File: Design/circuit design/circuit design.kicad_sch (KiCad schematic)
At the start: 22 parts, among them P1 USB_C_Plug_USB2.0, U1 STM32H743VITx, U2 NEO-7M-0, U3 ESP-01, U4 TP4056-42-ESOP8, U5 MP1584EN, U6 MP1584EN

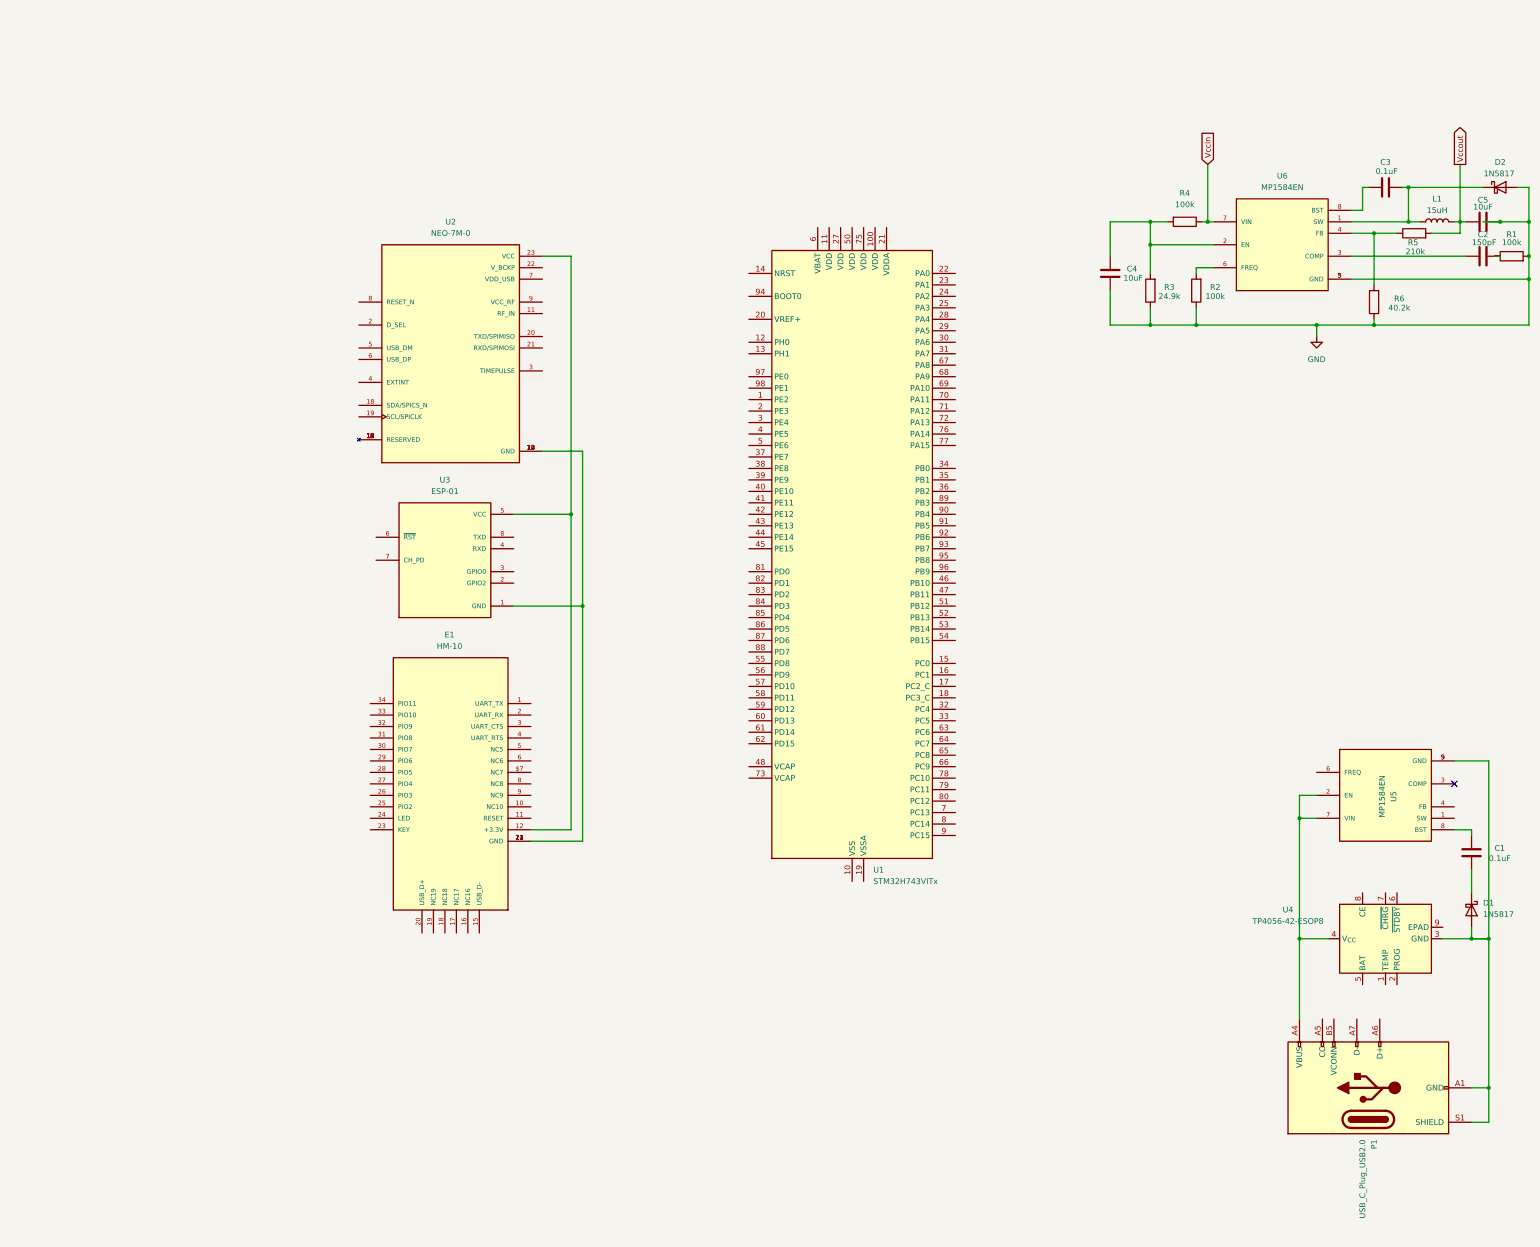
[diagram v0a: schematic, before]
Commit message: [2025-11-20 15:18:30 From Windows 11 Home]: Update
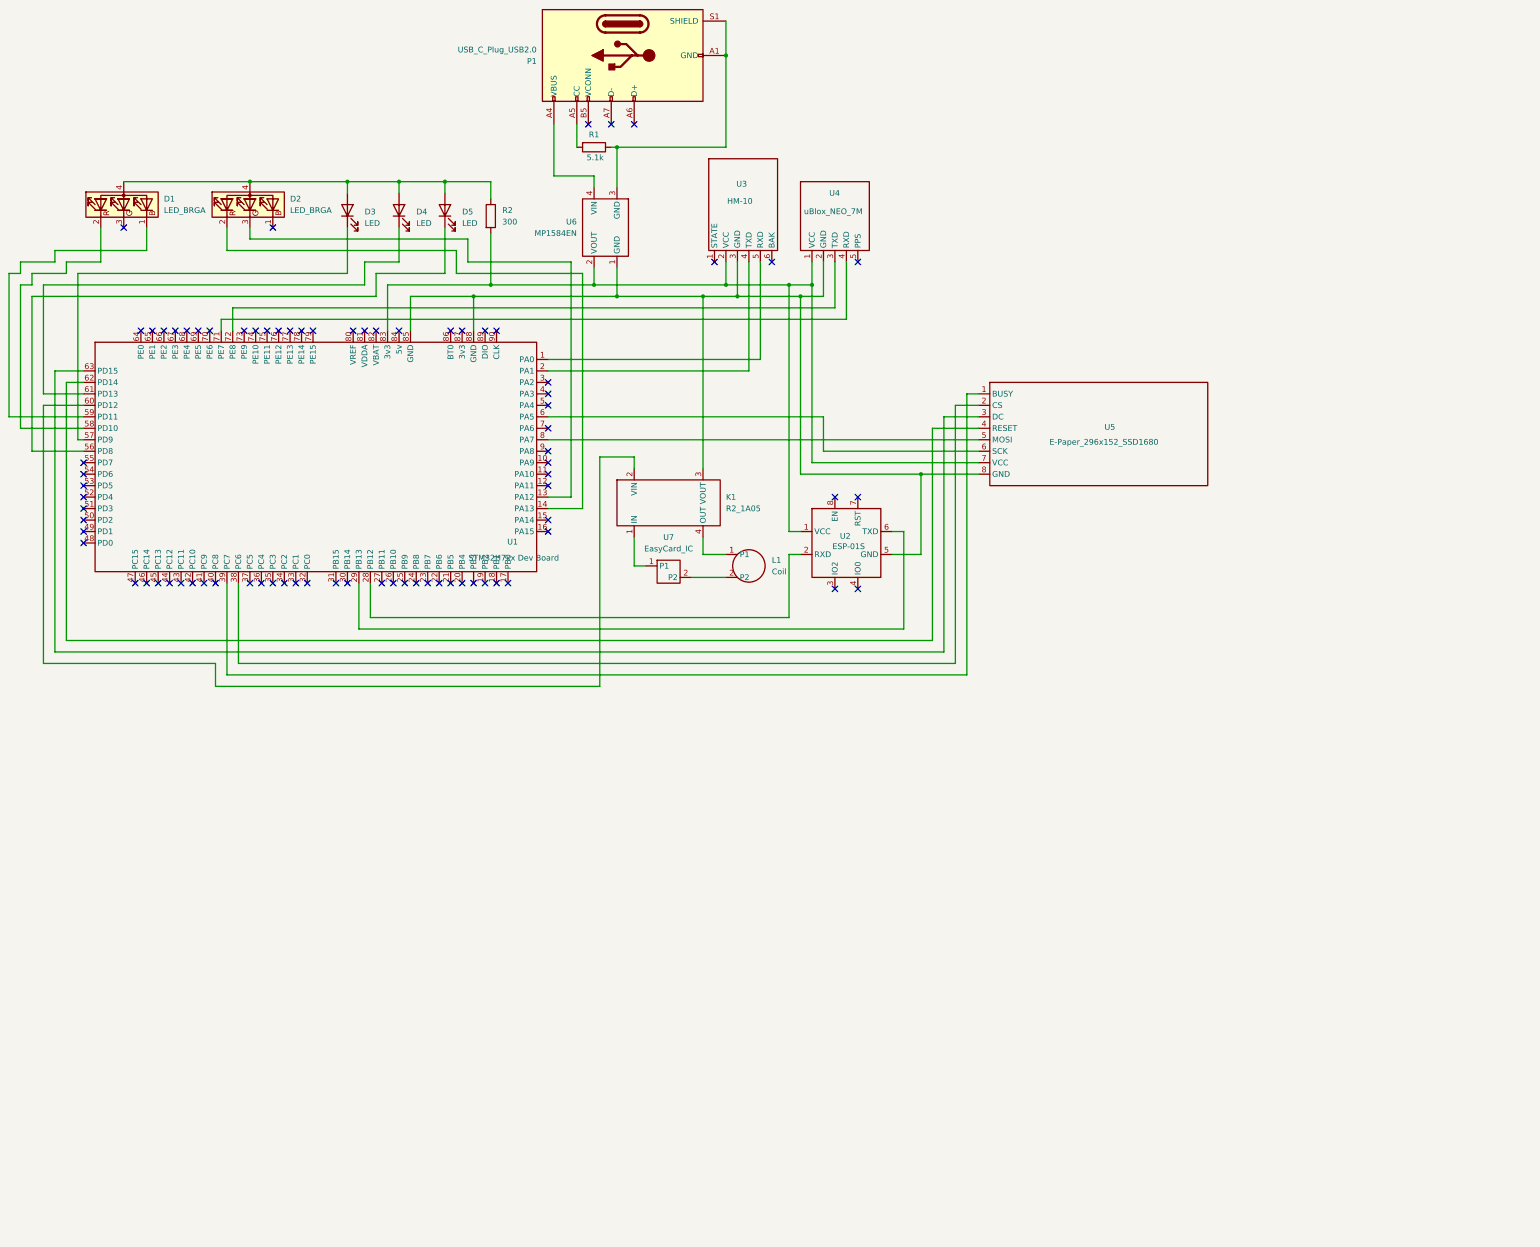
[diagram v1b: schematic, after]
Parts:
- removed C1, C3: 0.1uF, symbol Device:C
- removed C2: 150pF, symbol Device:C
- removed C4, C5: 10uF, symbol Device:C
- removed D1, D2: 1N5817, Diode_THT:D_DO-41_SOD81_P10.16mm_Horizontal, symbol Diode:1N5817
- removed E1: HM-10, HM-10:26.9X13X2.2_BOARD, symbol HM-10:HM-10
- removed L1: 15uH, symbol Device:L
- removed R3: 24.9k, symbol Device:R
- removed R4: 100k, symbol Device:R
- removed R5: 210k, symbol Device:R
- removed R6: 40.2k, symbol Device:R
- removed U1: STM32H743VITx, Package_QFP:LQFP-100_14x14mm_P0.5mm, symbol MCU_ST_STM32H7:STM32H743VITx
- removed U2: NEO-7M-0, NEO-7M-0:XCVR_NEO-7M-0, symbol NEO-7M-0:NEO-7M-0
- removed U3: ESP-01, ESP-01:MODULE_ESP-01, symbol ESP-01:ESP-01
- removed U4: TP4056-42-ESOP8, Package_SO:SOIC-8-1EP_3.9x4.9mm_P1.27mm_EP2.41x3.3mm_ThermalVias, symbol Battery_Management:TP4056-42-ESOP8
- removed U5, U6: MP1584EN, MP1584EN:SOIC127P600X170-9N, symbol MP1584EN:MP1584EN
- added D1, D2: LED_BRGA, symbol Device:LED_BRGA
- added D3, D4, D5: LED, symbol Device:LED
- added K1: R2_1A05, symbol New_Library:R2_1A05
- added L1: Coil, symbol New_Library:Coil
- added U1: STM32H7xx Dev Board, symbol New_Library:STM32H7_Dev_Board
- added U2: ESP-01S, symbol New_Library:ESP-01S_Module
- added U3: HM-10, symbol New_Library:HM-10_Module
- added U4: uBlox_NEO_7M, symbol New_Library:uBlox_NEO-7M_Module
- added U5: E-Paper_296x152_SSD1680, symbol New_Library:2.66'_E-Paper_SSD1680
- added U6: MP1584EN, symbol New_Library:MP1584EN_Module
- added U7: EasyCard_IC, symbol New_Library:EasyCard_IC
- R1: value 100k -> 5.1k
- R2: value 100k -> 300
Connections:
- net at P1.A1 (GND), P1.A12 (GND), P1.B1 (GND)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: now also R1.1, U6.3 (GND)
- net at P1.A4 (VBUS), P1.A9 (VBUS), P1.B4 (VBUS)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: now also U6.4 (VIN)
- net at R2.2: now also U1.83 (3v3), U2.1 (VCC), U3.2 (VCC), U4.1 (VCC), U5.7 (VCC), U6.2 (VOUT)
- net at P1.A5 (CC): now also R1.2
- net GND: no longer names the net of R2.1
- net GND: now also D1.4 (A), D2.4 (A), D3.2 (A), D4.2 (A), D5.2 (A); no longer R1.2
- new net: U1.39 (PC7), U5.1 (BUSY)
- new net: U1.38 (PC6), U5.2 (CS)
- new net: U1.63 (PD15), U5.3 (DC)
- new net: U1.62 (PD14), U5.4 (RESET)
- new net: U1.8 (PA7), U5.5 (MOSI)
- new net: U1.6 (PA5), U5.6 (SCK)
- new net: K1.3 (VOUT), U1.85 (GND), U1.88 (GND), U2.5 (GND), U3.3 (GND), U4.2 (GND), U5.8 (GND), U6.1 (GND)
- new net: D5.1 (K), U1.56 (PD8)
- new net: K1.4 (OUT), L1.1 (P1)
- new net: L1.2 (P2), U7.2 (P2)
- new net: U1.1 (PA0), U3.5 (RXD)
- new net: D2.3 (GK), U1.13 (PA12)
- new net: D2.2 (RK), U1.14 (PA13)
- new net: U1.2 (PA1), U3.4 (TXD)
- new net: U1.28 (PB12), U2.2 (RXD)
- new net: U1.29 (PB13), U2.6 (TXD)
- new net: D3.1 (K), U1.57 (PD9)
- new net: D1.2 (RK), U1.58 (PD10)
- new net: D1.1 (BK), U1.59 (PD11)
- new net: K1.2 (VIN), U1.60 (PD12)
- new net: D4.1 (K), U1.61 (PD13)
- new net: U1.71 (PE7), U4.4 (RXD)
- new net: U1.72 (PE8), U4.3 (TXD)
- new net: K1.1 (IN), U7.1 (P1)
- no-connect marks 1 -> 80
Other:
- company: (none) -> WUFAI
- title: (none) -> AI Wallet

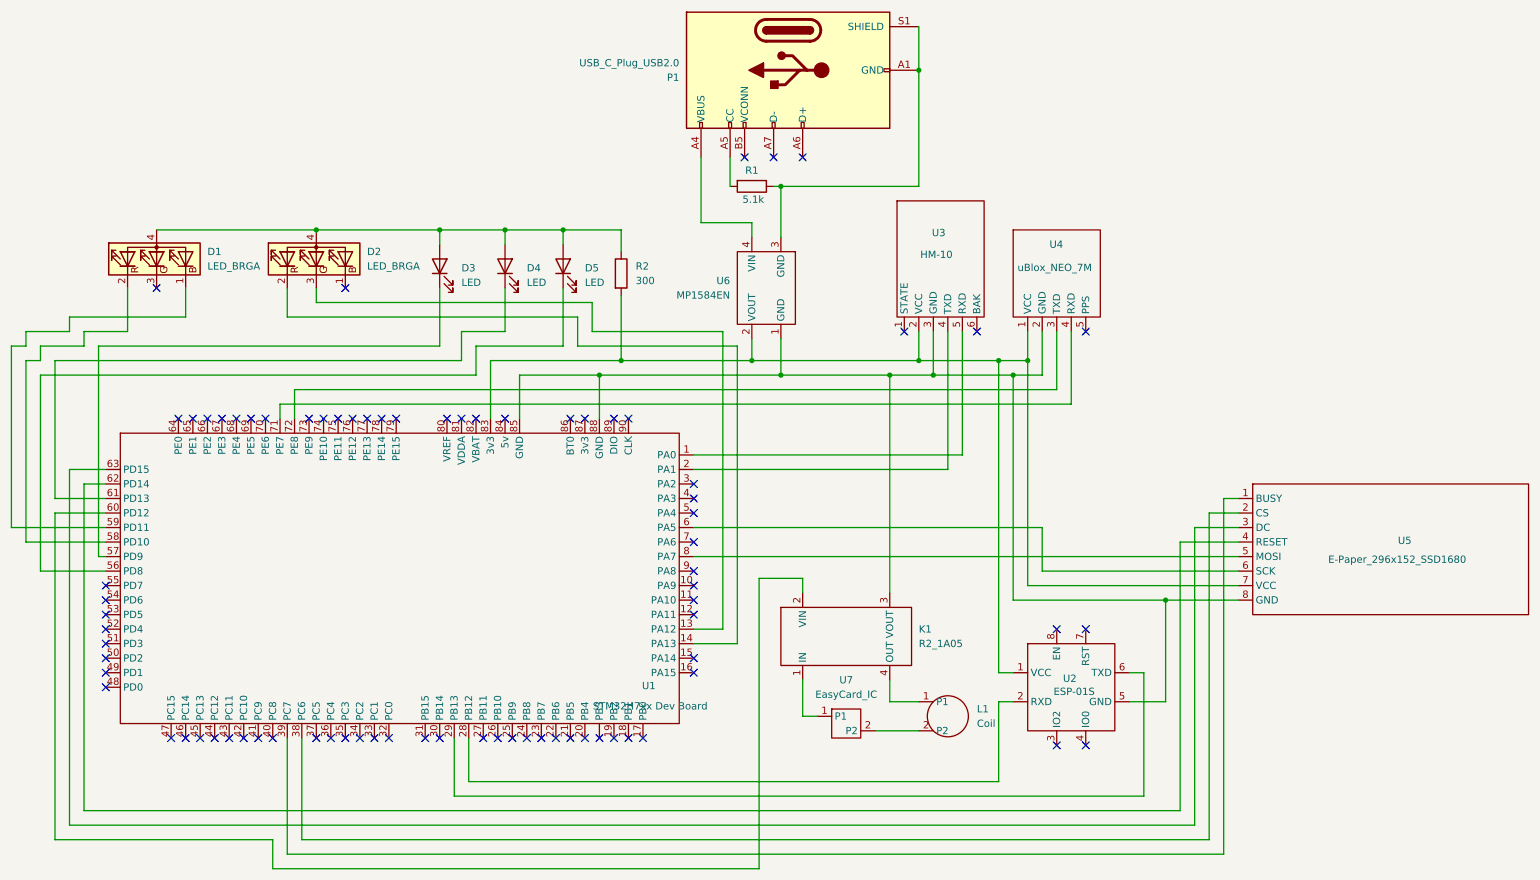
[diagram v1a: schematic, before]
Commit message: [2025-12-20 02:36:05 From Windows 11 Home]: Upadte
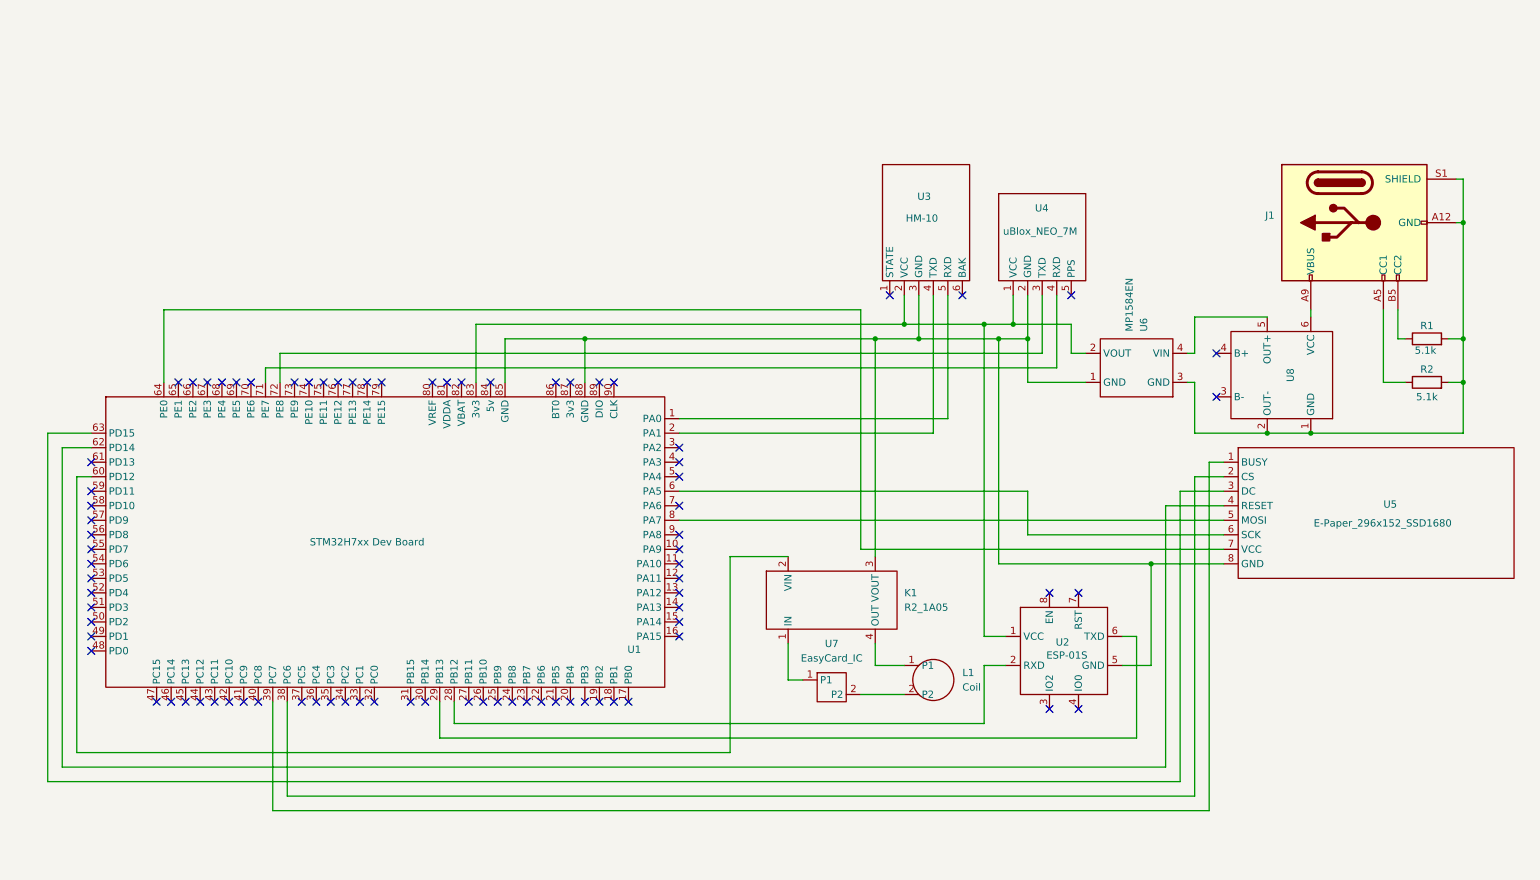
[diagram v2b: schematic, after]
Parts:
- removed D1, D2: LED_BRGA, symbol Device:LED_BRGA
- removed D3, D4, D5: LED, symbol Device:LED
- removed P1: USB_C_Plug_USB2.0, symbol Connector:USB_C_Plug_USB2.0
- added J1: USB_C_Receptacle_PowerOnly_6P, Connector_PinHeader_2.54mm:PinHeader_2x06_P2.54mm_Vertical, symbol Connector:USB_C_Receptacle_PowerOnly_6P
- added U8: TP4056, Module:TP4056, symbol New_Library:TP4056_Module
- K1: footprint (none) -> Package_DIP:DIP-14_W7.62mm_Socket
- L1: footprint (none) -> Connector_PinHeader_2.54mm:PinHeader_1x02_P2.54mm_Vertical
- R1: footprint (none) -> Resistor_THT:R_Axial_DIN0411_L9.9mm_D3.6mm_P12.70mm_Horizontal
- R2: value 300 -> 5.1k; footprint (none) -> Resistor_THT:R_Axial_DIN0411_L9.9mm_D3.6mm_P12.70mm_Horizontal
- U1: footprint (none) -> Module:MODULE_STM327H7xx Dev Module
- U2: footprint (none) -> Connector_PinHeader_2.54mm:PinHeader_2x04_P2.54mm_Vertical
- U3: footprint (none) -> Connector_PinHeader_2.54mm:PinHeader_1x06_P2.54mm_Vertical
- U4: footprint (none) -> Connector_PinHeader_2.54mm:PinHeader_1x05_P2.54mm_Vertical
- U5: footprint (none) -> Connector_PinHeader_2.54mm:PinHeader_1x08_P2.54mm_Vertical
- U6: footprint (none) -> Module:MP1584EN Module
- U7: footprint (none) -> Connector_PinHeader_2.54mm:PinHeader_1x03_P2.54mm_Vertical
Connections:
- net at U1.83 (3v3), U2.1 (VCC), U3.2 (VCC)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: no longer R2.2, U5.7 (VCC)
- net at R2.1: now also J1.A5 (CC1)
- net at U1.64 (PE0): now also U5.7 (VCC)
- net at U6.3 (GND): now also R1.2, R2.2, J1.A12 (GND), J1.B12 (GND), J1.S1 (SHIELD), U8.1 (GND), U8.2 (OUT-); no longer R1.1
- net at U6.4 (VIN): now also U8.5 (OUT+)
- new net: J1.A9 (VBUS), J1.B9 (VBUS), U8.6 (VCC)
- new net: J1.B5 (CC2), R1.1
- no-connect marks 80 -> 83
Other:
- moved on the sheet: K1, L1, U2, U3, U4, U5, U6, U7

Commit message: [2026-03-20 09:13:34 From Windows 11 Home]: Windows auto commit
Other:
- company: WUFAI -> WUFAI ELE 3B
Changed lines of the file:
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@@
 		(date "2025-11-14")
 		(rev "v1.0.0")
-		(company "WUFAI")
+		(company "WUFAI ELE 3B")
 	)
 	(junction
